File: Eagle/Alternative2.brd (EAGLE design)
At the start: 67 x 53 mm, 19 parts, among them IC2 PCA82C251, Q1 16MHz

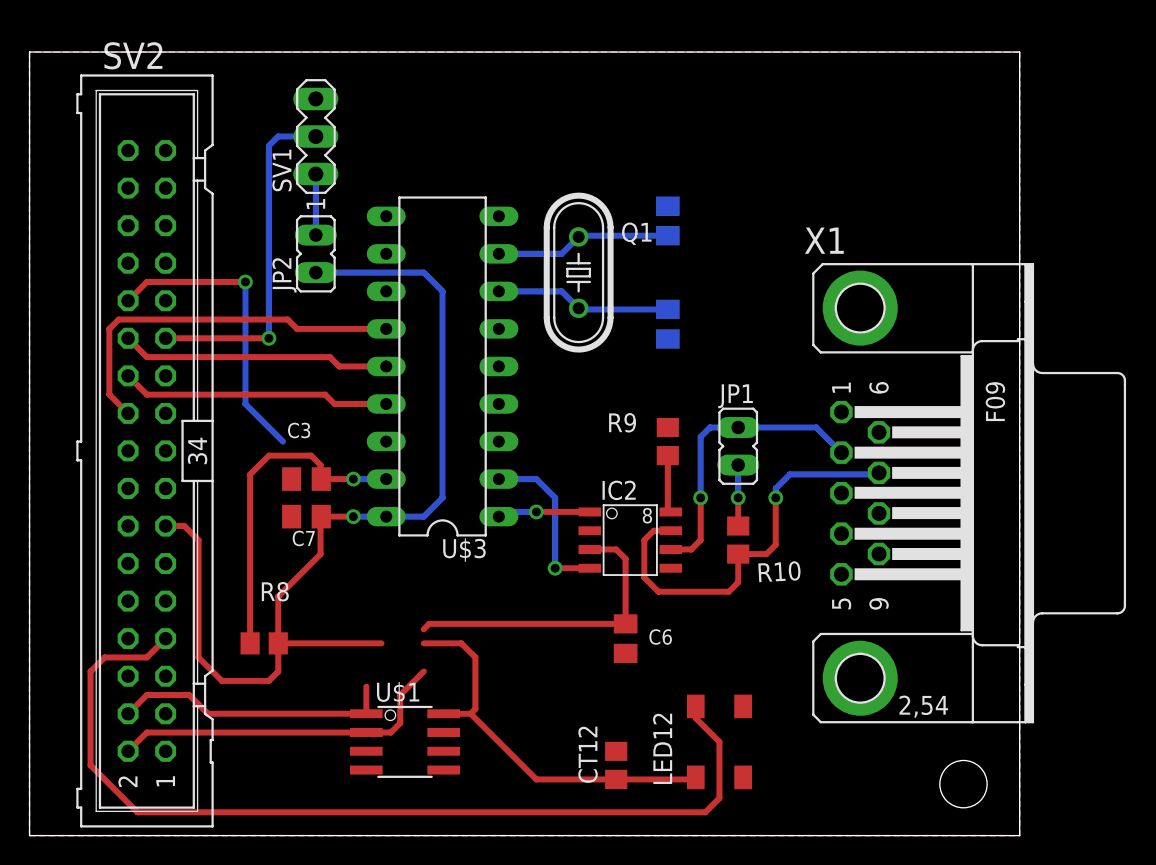
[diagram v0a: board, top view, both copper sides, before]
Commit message: update1 hw review
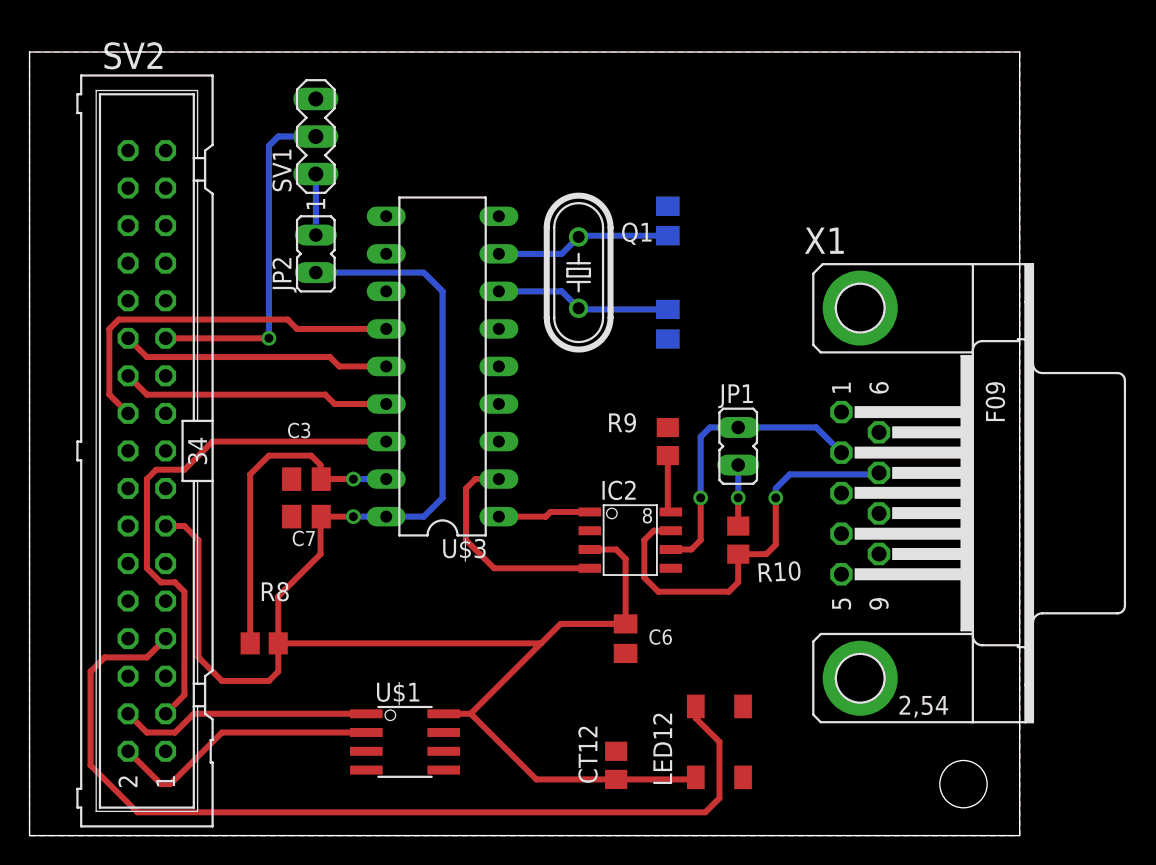
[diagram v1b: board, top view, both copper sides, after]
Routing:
- net PD0: track 0.00 -> 35.3 mm
- net PB2: track 20.3 -> 0.00 mm, vias 1 -> 0
- net PC5: track 23.4 -> 18.5 mm
- net N$6: track 11.4 -> 15.1 mm, vias 1 -> 0
- net PC4: track 19.0 -> 17.2 mm
- net +5V: track 115.0 -> 116.5 mm
- net N$7: vias 1 -> 0
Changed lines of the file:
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@@
 <contactref element="CT12" pad="1"/>
 <contactref element="U$1" pad="8"/>
-<wire x1="30.1625" y1="8.5725" x2="30.1625" y2="12.065" width="0.4064" layer="1"/>
-<wire x1="30.1625" y1="12.065" x2="29.21" y2="13.0175" width="0.4064" layer="1"/>
-<wire x1="29.21" y1="13.0175" x2="26.6725" y2="13.0175" width="0.4064" layer="1"/>
 <wire x1="39.6875" y1="3.8125" x2="44.935" y2="3.8125" width="0.4064" layer="1"/>
 <wire x1="44.935" y1="3.8125" x2="45.0725" y2="3.95" width="0.4064" layer="1"/>
@@
 <contactref element="U$3" pad="18"/>
 <wire x1="28.0162" y1="8.255" x2="29.845" y2="8.255" width="0.4064" layer="1"/>
-<wire x1="29.845" y1="8.255" x2="30.1625" y2="8.5725" width="0.4064" layer="1"/>
 <wire x1="39.6875" y1="3.8125" x2="34.2875" y2="3.8125" width="0.4064" layer="1"/>
 <wire x1="34.2875" y1="3.8125" x2="29.845" y2="8.255" width="0.4064" layer="1"/>
@@
 <wire x1="19.685" y1="19.05" x2="19.685" y2="21.5425" width="0.4064" layer="1"/>
 <wire x1="19.685" y1="21.5425" x2="19.7325" y2="21.59" width="0.4064" layer="1"/>
-<wire x1="16.825" y1="13.0175" x2="23.81" y2="13.0175" width="0.4064" layer="1"/>
 <wire x1="37.8968" y1="19.3675" x2="39.6875" y2="19.3675" width="0.4064" layer="1"/>
 <wire x1="39.6875" y1="19.3675" x2="40.3225" y2="18.7325" width="0.4064" layer="1"/>
 <wire x1="40.3225" y1="18.7325" x2="40.3225" y2="14.335" width="0.4064" layer="1"/>
-<wire x1="40.3225" y1="14.335" x2="27.035" y2="14.335" width="0.4064" layer="1"/>
-<wire x1="27.035" y1="14.335" x2="26.67" y2="13.97" width="0.4064" layer="1"/>
-<wire x1="26.6725" y1="13.0175" x2="26.67" y2="13.97" width="0" layer="19" extent="1-1"/>
-<wire x1="23.81" y1="13.0175" x2="26.6725" y2="13.0175" width="0" layer="19" extent="1-1"/>
+<wire x1="40.3225" y1="14.335" x2="35.925" y2="14.335" width="0.4064" layer="1"/>
+<wire x1="35.925" y1="14.335" x2="34.6075" y2="13.0175" width="0.4064" layer="1"/>
+<wire x1="34.6075" y1="13.0175" x2="29.845" y2="8.255" width="0.4064" layer="1"/>
+<wire x1="17.4625" y1="13.0175" x2="34.6075" y2="13.0175" width="0.4064" layer="1"/>
+<wire x1="16.825" y1="13.0175" x2="17.4625" y2="13.0175" width="0" layer="19" extent="1-1"/>
 </signal>
 <signal name="PB3">
@@
 <contactref element="SV2" pad="4"/>
 <contactref element="U$1" pad="1"/>
-<wire x1="22.7838" y1="8.255" x2="22.7838" y2="10.0863" width="0.4064" layer="1"/>
-<wire x1="22.7838" y1="8.255" x2="12.065" y2="8.255" width="0.4064" layer="1"/>
-<wire x1="12.065" y1="8.255" x2="10.795" y2="9.525" width="0.4064" layer="1"/>
-<wire x1="10.795" y1="9.525" x2="7.9375" y2="9.525" width="0.4064" layer="1"/>
-<wire x1="7.9375" y1="9.525" x2="6.6675" y2="8.255" width="0.4064" layer="1"/>
+<wire x1="22.7838" y1="8.255" x2="11.1125" y2="8.255" width="0.4064" layer="1"/>
+<wire x1="11.1125" y1="8.255" x2="9.8425" y2="6.985" width="0.4064" layer="1"/>
+<wire x1="9.8425" y1="6.985" x2="7.9375" y2="6.985" width="0.4064" layer="1"/>
+<wire x1="7.9375" y1="6.985" x2="6.6675" y2="8.255" width="0.4064" layer="1"/>
 </signal>
 <signal name="PC5">
 <contactref element="SV2" pad="2"/>
 <contactref element="U$1" pad="2"/>
-<wire x1="6.6675" y1="5.715" x2="7.9375" y2="6.985" width="0.4064" layer="1"/>
-<wire x1="7.9375" y1="6.985" x2="22.7838" y2="6.985" width="0.4064" layer="1"/>
-<wire x1="26.67" y1="11.1125" x2="25.0825" y2="9.525" width="0.4064" layer="1"/>
-<wire x1="25.0825" y1="9.525" x2="25.0825" y2="7.62" width="0.4064" layer="1"/>
-<wire x1="25.0825" y1="7.62" x2="24.4475" y2="6.985" width="0.4064" layer="1"/>
-<wire x1="24.4475" y1="6.985" x2="22.7838" y2="6.985" width="0.4064" layer="1"/>
+<wire x1="22.7838" y1="6.985" x2="13.0175" y2="6.985" width="0.4064" layer="1"/>
+<wire x1="13.0175" y1="6.985" x2="9.525" y2="3.4925" width="0.4064" layer="1"/>
+<wire x1="9.525" y1="3.4925" x2="8.89" y2="3.4925" width="0.4064" layer="1"/>
+<wire x1="8.89" y1="3.4925" x2="6.6675" y2="5.715" width="0.4064" layer="1"/>
 </signal>
 <signal name="N$4">
@@
 <contactref element="IC2" pad="4"/>
 <contactref element="U$3" pad="2"/>
-<wire x1="37.8968" y1="18.0975" x2="35.56" y2="18.0975" width="0.4064" layer="1"/>
-<via x="35.56" y="18.0975" extent="1-16" drill="0.6" shape="square"/>
-<wire x1="35.56" y1="18.0975" x2="35.56" y2="22.86" width="0.4064" layer="16"/>
-<wire x1="35.56" y1="22.86" x2="34.29" y2="24.13" width="0.4064" layer="16"/>
-<wire x1="34.29" y1="24.13" x2="31.75" y2="24.13" width="0.4064" layer="16"/>
+<wire x1="37.8968" y1="18.0975" x2="31.4325" y2="18.0975" width="0.4064" layer="1"/>
+<wire x1="31.4325" y1="18.0975" x2="29.5275" y2="20.0025" width="0.4064" layer="1"/>
+<wire x1="29.5275" y1="20.0025" x2="29.5275" y2="23.495" width="0.4064" layer="1"/>
+<wire x1="29.5275" y1="23.495" x2="30.1625" y2="24.13" width="0.4064" layer="1"/>
+<wire x1="30.1625" y1="24.13" x2="31.75" y2="24.13" width="0.4064" layer="1"/>
 </signal>
 <signal name="N$7">
 <contactref element="IC2" pad="1"/>
 <contactref element="U$3" pad="1"/>
-<wire x1="37.8968" y1="21.9075" x2="34.29" y2="21.9075" width="0.4064" layer="1"/>
-<via x="34.29" y="21.9075" extent="1-16" drill="0.6" shape="square"/>
-<wire x1="34.29" y1="21.9075" x2="32.0675" y2="21.9075" width="0.4064" layer="16"/>
-<wire x1="32.0675" y1="21.9075" x2="31.75" y2="21.59" width="0.4064" layer="16"/>
+<wire x1="37.8968" y1="21.9075" x2="35.2425" y2="21.9075" width="0.4064" layer="1"/>
+<wire x1="35.2425" y1="21.9075" x2="34.925" y2="21.59" width="0.4064" layer="1"/>
+<wire x1="34.925" y1="21.59" x2="31.75" y2="21.59" width="0.4064" layer="1"/>
 </signal>
 <signal name="N$8">
@@
 <contactref element="SV2" pad="3"/>
 <contactref element="U$3" pad="16"/>
-<wire x1="9.2075" y1="8.255" x2="24.13" y2="26.67" width="0" layer="19" extent="1-1"/>
+<wire x1="24.13" y1="26.67" x2="12.3825" y2="26.67" width="0.4064" layer="1"/>
+<wire x1="12.3825" y1="26.67" x2="10.4775" y2="24.765" width="0.4064" layer="1"/>
+<wire x1="10.4775" y1="24.765" x2="8.5725" y2="24.765" width="0.4064" layer="1"/>
+<wire x1="8.5725" y1="24.765" x2="7.9375" y2="24.13" width="0.4064" layer="1"/>
+<wire x1="7.9375" y1="24.13" x2="7.9375" y2="18.0975" width="0.4064" layer="1"/>
+<wire x1="7.9375" y1="18.0975" x2="8.89" y2="17.145" width="0.4064" layer="1"/>
+<wire x1="8.89" y1="17.145" x2="9.8425" y2="17.145" width="0.4064" layer="1"/>
+<wire x1="9.8425" y1="17.145" x2="10.4775" y2="16.51" width="0.4064" layer="1"/>
+<wire x1="10.4775" y1="16.51" x2="10.4775" y2="9.525" width="0.4064" layer="1"/>
+<wire x1="10.4775" y1="9.525" x2="9.2075" y2="8.255" width="0.4064" layer="1"/>
 </signal>
 <signal name="PD1">
@@
 <signal name="PB2">
 <contactref element="SV2" pad="26"/>
-<wire x1="6.6675" y1="36.195" x2="7.9375" y2="37.465" width="0.4064" layer="1"/>
-<wire x1="7.9375" y1="37.465" x2="14.605" y2="37.465" width="0.4064" layer="1"/>
-<via x="14.605" y="37.465" extent="1-16" drill="0.6" shape="square"/>
-<wire x1="14.605" y1="37.465" x2="14.605" y2="29.21" width="0.4064" layer="16"/>
-<wire x1="14.605" y1="29.21" x2="17.145" y2="26.67" width="0.4064" layer="16"/>
 </signal>
 <signal name="N$16">

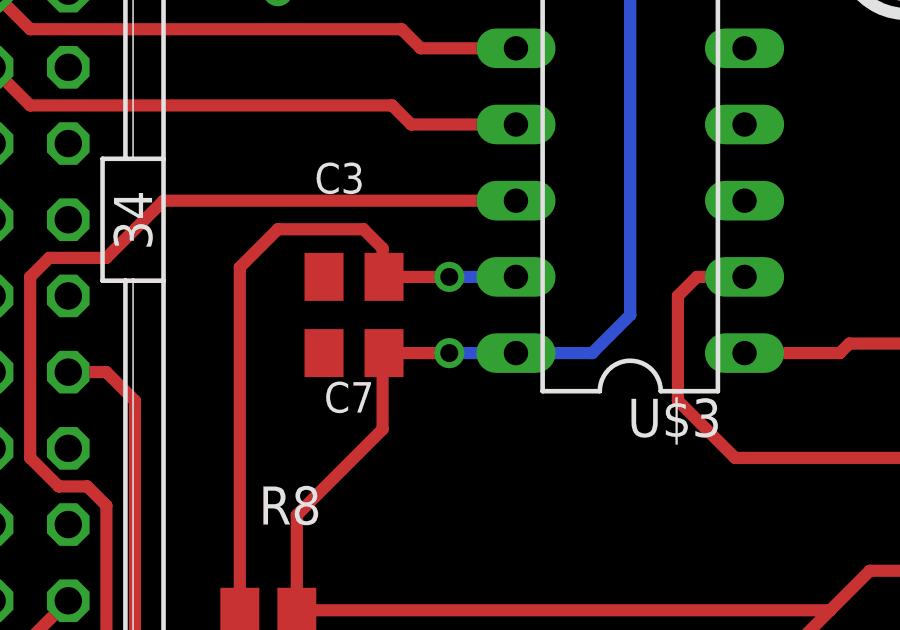
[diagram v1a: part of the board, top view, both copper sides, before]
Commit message: Update2
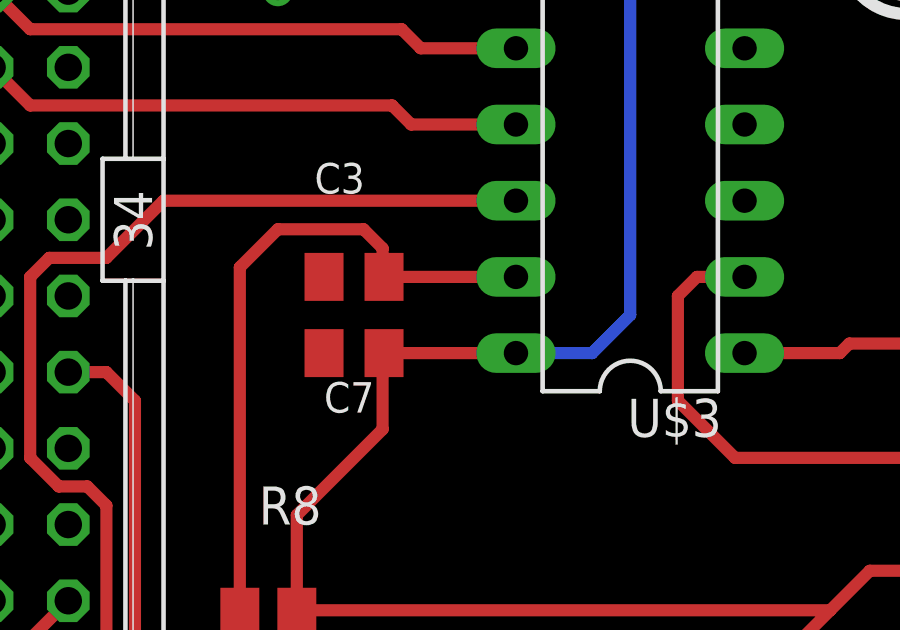
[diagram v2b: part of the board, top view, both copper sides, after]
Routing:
- net +5V: vias 1 -> 0
- net N$4: vias 1 -> 0
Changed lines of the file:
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@@
 <wire x1="27.94" y1="36.83" x2="26.67" y2="38.1" width="0.4064" layer="16"/>
 <wire x1="26.67" y1="38.1" x2="19.3675" y2="38.1" width="0.4064" layer="16"/>
-<wire x1="24.13" y1="21.59" x2="21.9075" y2="21.59" width="0.4064" layer="16"/>
-<via x="21.9075" y="21.59" extent="1-16" drill="0.6" shape="square"/>
-<wire x1="21.9075" y1="21.59" x2="19.7325" y2="21.59" width="0.4064" layer="1"/>
 <wire x1="16.825" y1="13.0175" x2="16.825" y2="16.19" width="0.4064" layer="1"/>
 <wire x1="16.825" y1="16.19" x2="19.685" y2="19.05" width="0.4064" layer="1"/>
@@
 <wire x1="34.6075" y1="13.0175" x2="29.845" y2="8.255" width="0.4064" layer="1"/>
 <wire x1="17.4625" y1="13.0175" x2="34.6075" y2="13.0175" width="0.4064" layer="1"/>
+<wire x1="19.7325" y1="21.59" x2="24.13" y2="21.59" width="0.4064" layer="1"/>
 <wire x1="16.825" y1="13.0175" x2="17.4625" y2="13.0175" width="0" layer="19" extent="1-1"/>
 </signal>
@@
 <wire x1="19.685" y1="25.0825" x2="19.685" y2="24.1775" width="0.4064" layer="1"/>
 <wire x1="19.685" y1="24.1775" x2="19.7325" y2="24.13" width="0.4064" layer="1"/>
-<wire x1="24.13" y1="24.13" x2="21.9075" y2="24.13" width="0.4064" layer="16"/>
-<via x="21.9075" y="24.13" extent="1-16" drill="0.6" shape="square"/>
-<wire x1="21.9075" y1="24.13" x2="19.7325" y2="24.13" width="0.4064" layer="1"/>
+<wire x1="19.7325" y1="24.13" x2="24.13" y2="24.13" width="0.4064" layer="1"/>
 </signal>
 <signal name="N$5">
